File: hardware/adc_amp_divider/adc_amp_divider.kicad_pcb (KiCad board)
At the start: 2 copper layers, 76.2 x 52.7 mm, 121 parts, among them M200 CONN_1, M201 CONN_1, M202 CONN_1, P201 CONN_10X2, P202 CONN_3, P203 CONN_2, P204 CONN_1, P205 CONN_1, P206 CONN_3, P207 CONN_2, P208 CONN_6, P209 CONN_6, U201 LMV324IDR, U202 LMV324IDR, U203 LMV324IDR

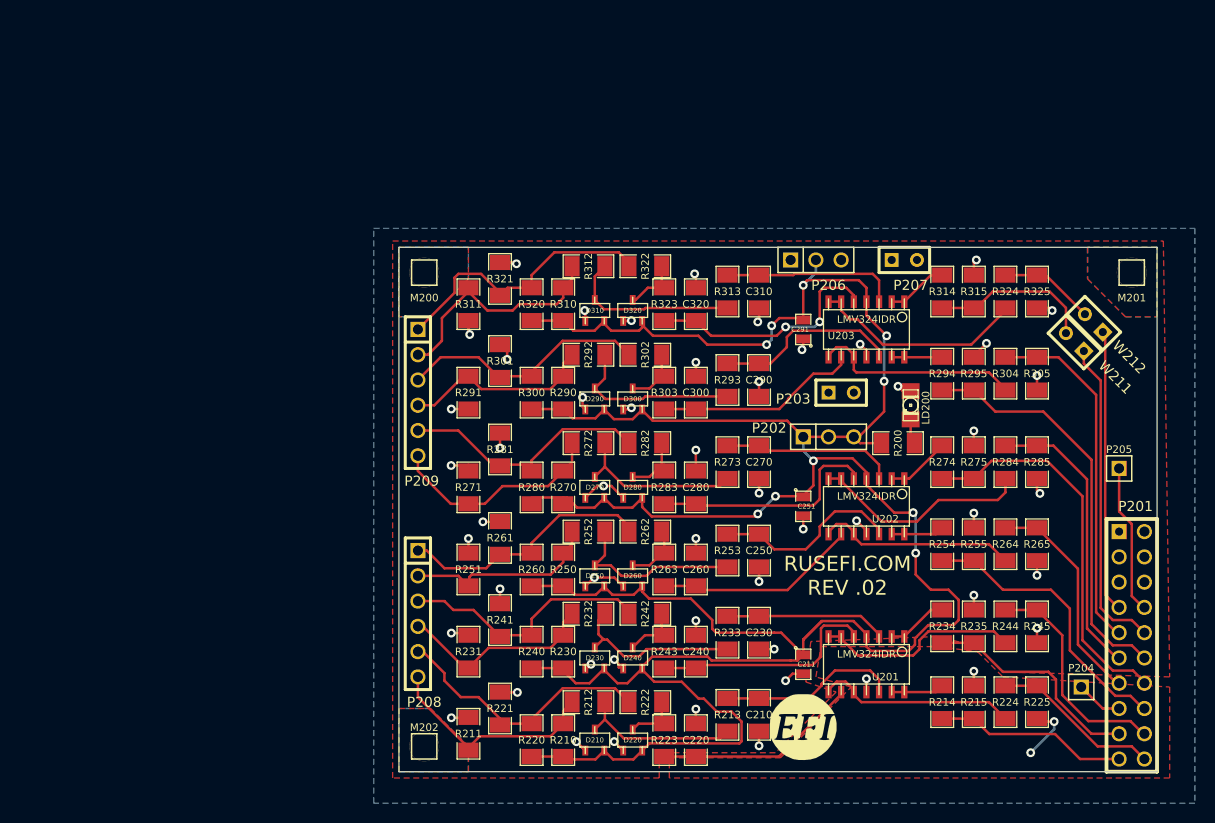
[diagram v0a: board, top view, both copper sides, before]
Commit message: proper location
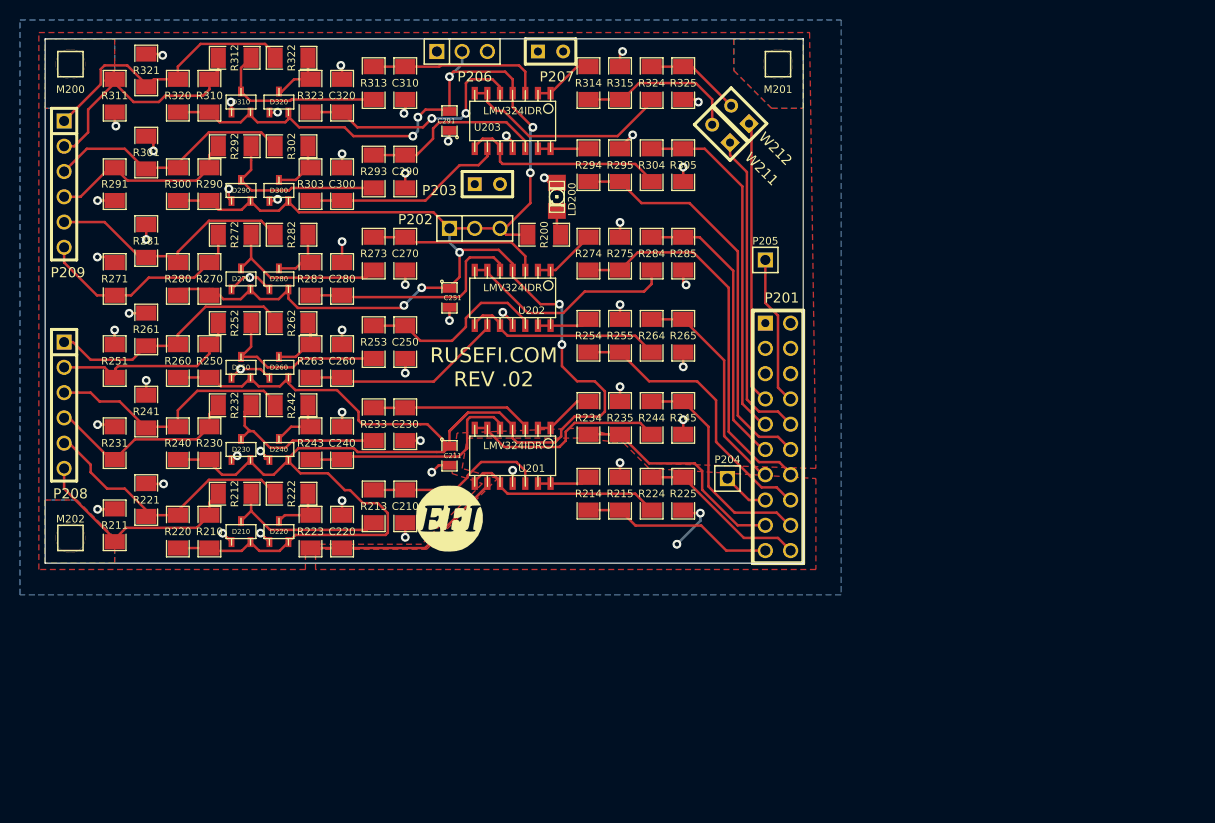
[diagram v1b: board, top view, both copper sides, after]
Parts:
- moved P206 41.3 mm to (96.5, 99.7)
- moved R295 41.3 mm to (112.4, 111.1)
- moved C240 41.3 mm to (84.5, 139.1)
- moved C300 41.3 mm to (84.5, 113.0)
- moved D230 41.3 mm to (74.3, 139.7)
- moved D240 41.3 mm to (78.1, 139.7)
- moved D250 41.3 mm to (74.3, 131.4)
- moved D260 41.3 mm to (78.1, 131.4)
- moved P203 41.3 mm to (99.1, 113.0)
- moved P207 41.3 mm to (105.4, 99.7)
- moved P208 41.3 mm to (56.5, 135.3)
- moved P209 41.3 mm to (56.5, 113.0)
- moved R211 41.3 mm to (61.6, 147.3)
- moved R213 41.3 mm to (87.6, 145.4)
- moved R221 41.3 mm to (64.8, 144.8)
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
